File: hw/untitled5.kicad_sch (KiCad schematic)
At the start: 6 parts, among them U2 LD39200, U6 TS3USB3031

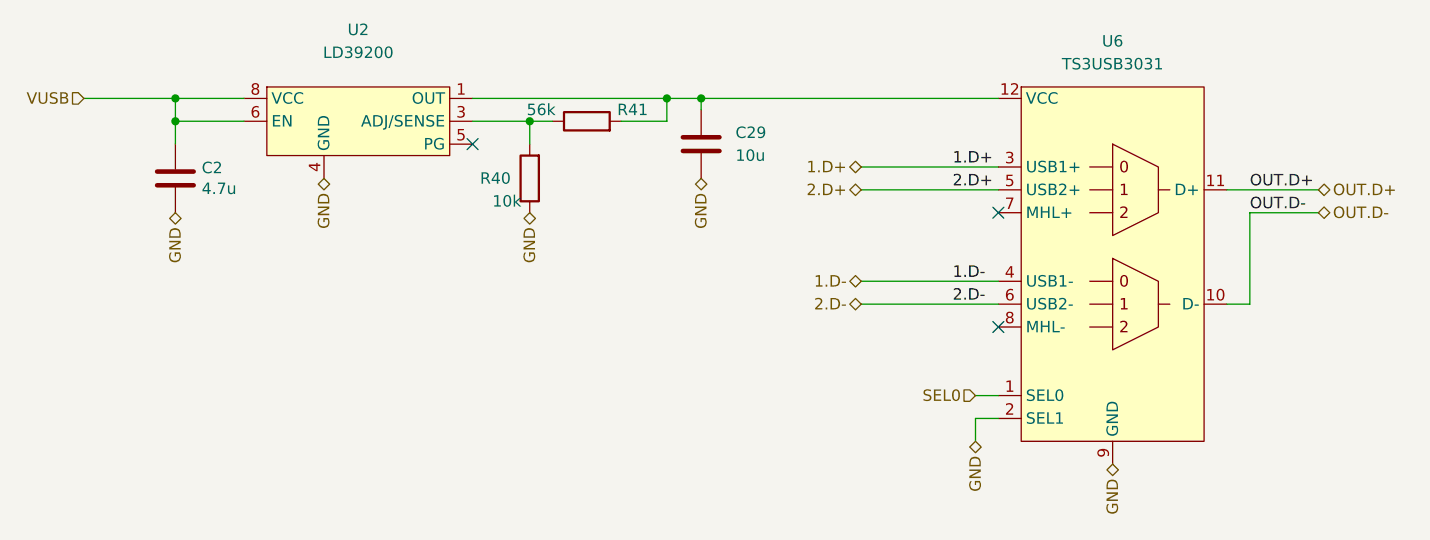
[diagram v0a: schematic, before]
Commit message: Inspection of parts complete
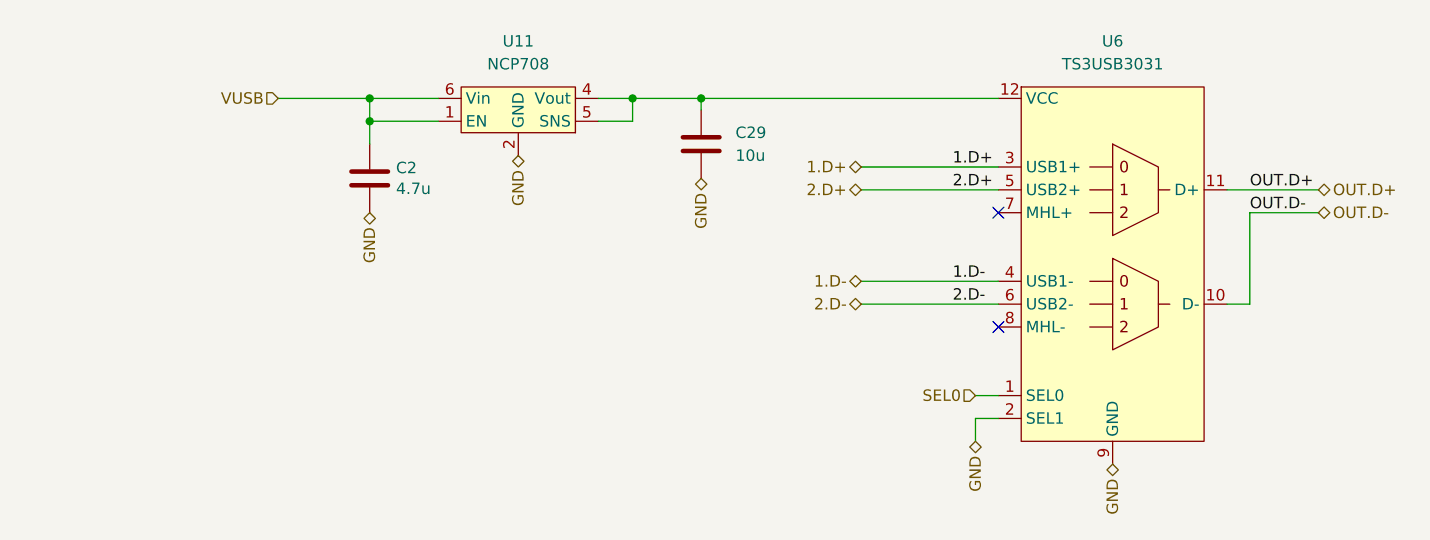
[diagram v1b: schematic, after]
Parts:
- removed R40: 10k, Resistor_SMD:R_0402_1005Metric, symbol Device:R
- removed R41: 56k, Resistor_SMD:R_0402_1005Metric, symbol Device:R
- removed U2: LD39200, Package_DFN_QFN:DFN-8-1EP_4x4mm_P0.8mm_EP2.3x3.24mm, symbol RKL-LDO:LD39200
- added U11: NCP708, RKL-StandardPackages:UDFN6-3x3mm, symbol RKL-LDO:NCP708
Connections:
- net GND: now also U11.2 (GND), U11.7 (GND)
- net at C29.1, U6.12 (VCC): now also U11.4 (Vout), U11.5 (SNS)
- net VCC renamed VUSB
- net VUSB: now also U11.1 (EN), U11.6 (Vin)
- no-connect marks 3 -> 2
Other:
- moved on the sheet: C2
